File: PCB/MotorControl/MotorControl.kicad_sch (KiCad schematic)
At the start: 14 parts, among them J1 USB_C_Receptacle_USB2.0_14P, J2 Conn_02x05_Top_Bottom, J3 Conn_01x06, J4 Conn_01x03, SW1 SW_Push, U1 STM32L031K6Tx, U2 TC1262-33

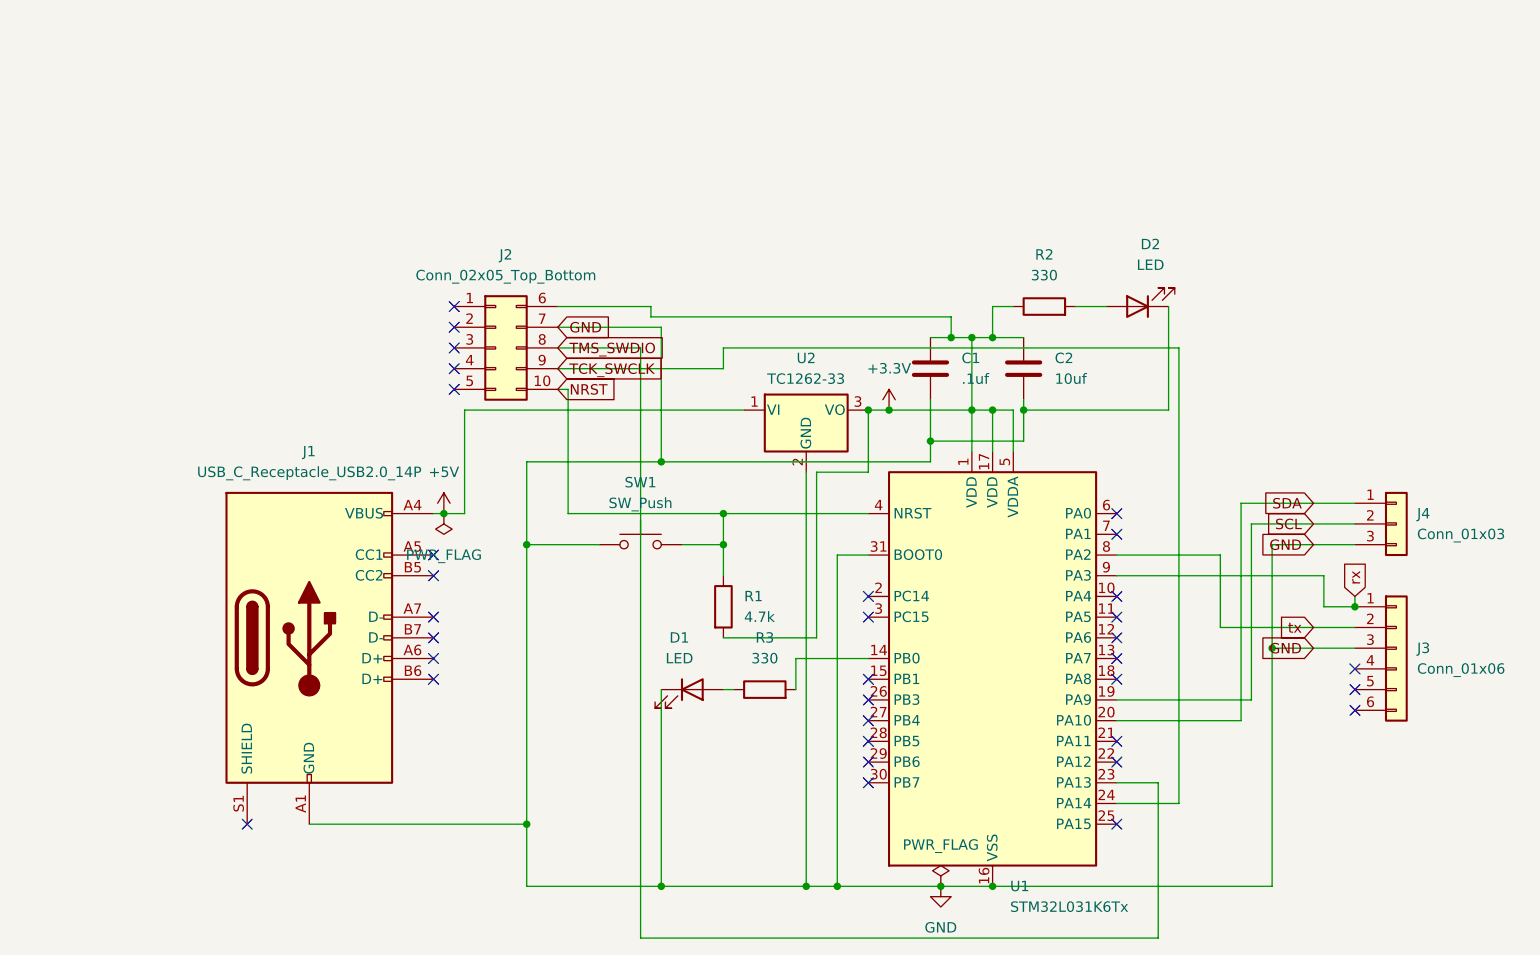
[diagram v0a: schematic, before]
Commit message: wasd
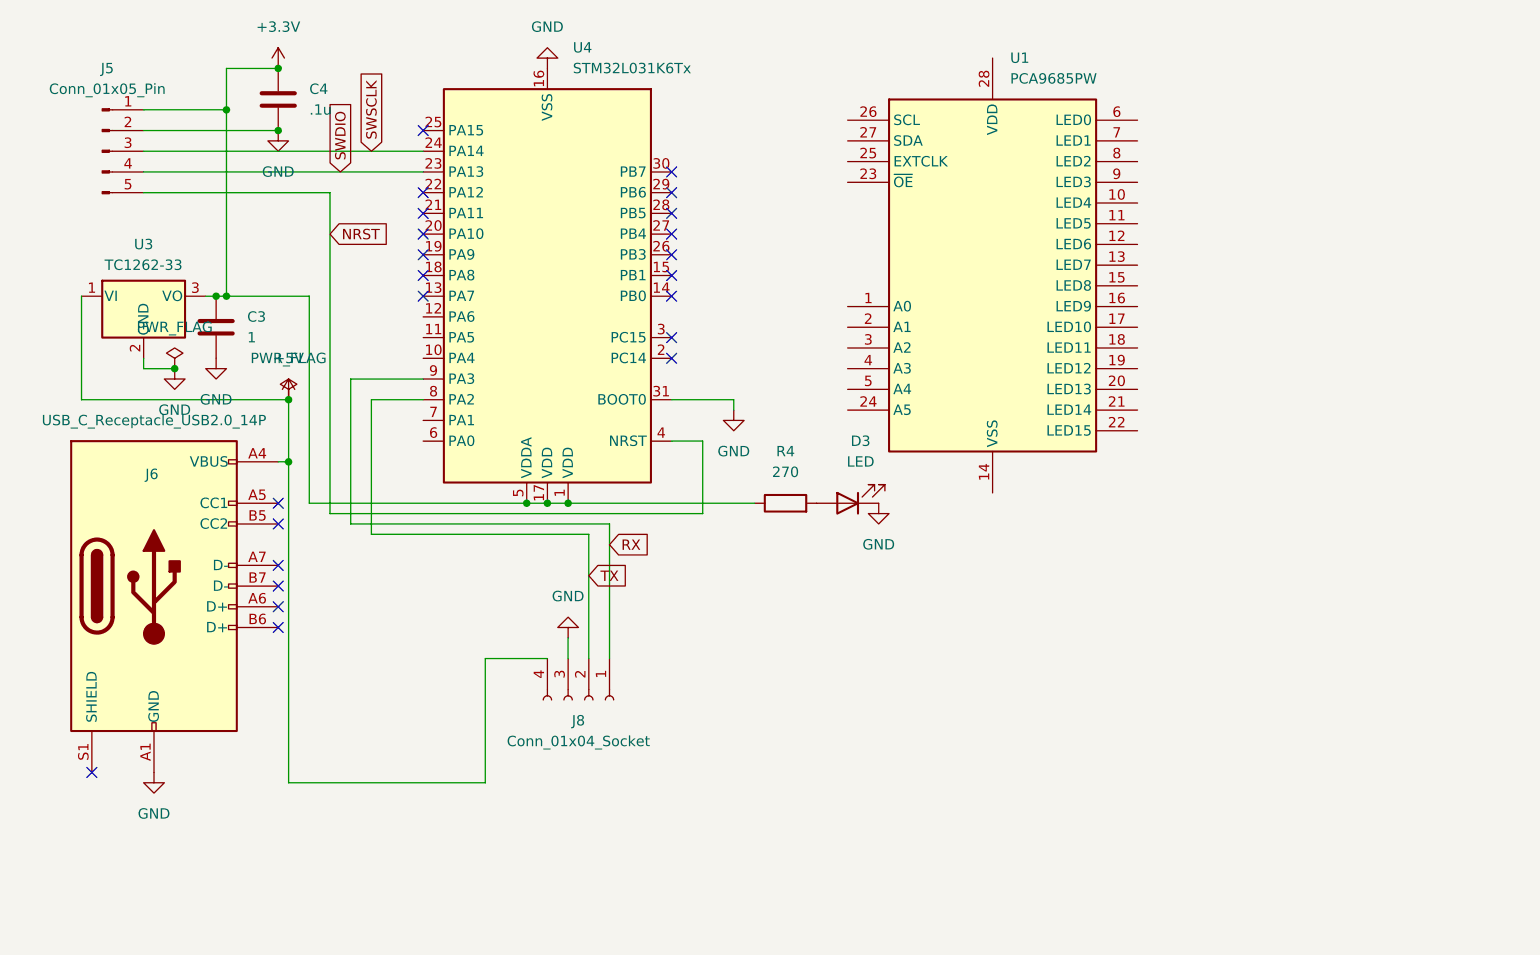
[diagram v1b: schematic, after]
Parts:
- removed C1: .1uf, Capacitor_SMD:C_0805_2012Metric_Pad1.18x1.45mm_HandSolder, symbol Device:C
- removed C2: 10uf, Capacitor_SMD:C_0805_2012Metric_Pad1.18x1.45mm_HandSolder, symbol Device:C
- removed D1, D2: LED, LED_SMD:LED_0805_2012Metric_Pad1.15x1.40mm_HandSolder, symbol Device:LED
- removed J1: USB_C_Receptacle_USB2.0_14P, Connector_USB:USB_C_Receptacle_GCT_USB4085, symbol Connector:USB_C_Receptacle_USB2.0_14P
- removed J2: Conn_02x05_Top_Bottom, Connector_PinHeader_2.54mm:PinHeader_2x05_P2.54mm_Vertical, symbol Connector_Generic:Conn_02x05_Top_Bottom
- removed J3: Conn_01x06, Connector_PinHeader_2.54mm:PinHeader_1x06_P2.54mm_Vertical, symbol Connector_Generic:Conn_01x06
- removed J4: Conn_01x03, Connector_PinHeader_2.54mm:PinHeader_1x03_P2.54mm_Vertical, symbol Connector_Generic:Conn_01x03
- removed R1: 4.7k, Resistor_SMD:R_0805_2012Metric_Pad1.20x1.40mm_HandSolder, symbol Device:R
- removed R2, R3: 330, Resistor_SMD:R_0805_2012Metric_Pad1.20x1.40mm_HandSolder, symbol Device:R
- removed SW1: SW_Push, Button_Switch_THT:SW_PUSH_6mm_H4.3mm, symbol Switch:SW_Push
- removed U1: STM32L031K6Tx, Package_QFP:LQFP-32_7x7mm_P0.8mm, symbol MCU_ST_STM32L0:STM32L031K6Tx
- removed U2: TC1262-33, Package_TO_SOT_SMD:SOT-223-3_TabPin2, symbol Regulator_Linear:TC1262-33
- added C3: 1, Capacitor_SMD:C_0504_1310Metric_Pad0.83x1.28mm_HandSolder, symbol Device:C
- added C4: .1u, Capacitor_SMD:C_0504_1310Metric_Pad0.83x1.28mm_HandSolder, symbol Device:C
- added D3: LED, LED_SMD:LED_1206_3216Metric_Pad1.42x1.75mm_HandSolder, symbol Device:LED
- added J5: Conn_01x05_Pin, Connector_PinHeader_1.00mm:PinHeader_1x05_P1.00mm_Vertical, symbol Connector:Conn_01x05_Pin
- added J6: USB_C_Receptacle_USB2.0_14P, Connector_USB:USB_C_Receptacle_GCT_USB4085, symbol Connector:USB_C_Receptacle_USB2.0_14P
- added J8: Conn_01x04_Socket, Connector_PinHeader_1.00mm:PinHeader_1x04_P1.00mm_Horizontal, symbol Connector:Conn_01x04_Socket
- added R4: 270, Resistor_SMD:R_0805_2012Metric_Pad1.20x1.40mm_HandSolder, symbol Device:R
- added U1: PCA9685PW, Package_SO:TSSOP-28_4.4x9.7mm_P0.65mm, symbol Driver_LED:PCA9685PW
- added U3: TC1262-33, Package_TO_SOT_SMD:SOT-223-3_TabPin2, symbol Regulator_Linear:TC1262-33
- added U4: STM32L031K6Tx, Package_QFP:LQFP-32_7x7mm_P0.8mm, symbol MCU_ST_STM32L0:STM32L031K6Tx
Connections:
- net +3.3V: now also C3.1, C4.1, J5.1 (Pin_1), R4.1, U3.3 (VO), U4.1 (VDD), U4.17 (VDD), U4.5 (VDDA)
- net +5V: now also J6.A4 (VBUS), J6.A9 (VBUS), J6.B4 (VBUS), J6.B9 (VBUS), J8.4 (Pin_4), U3.1 (VI)
- net GND: now also C3.2, C4.2, D3.1 (K), J5.2 (Pin_2), J6.A1 (GND), J6.A12 (GND), J6.B1 (GND), J6.B12 (GND), J8.3 (Pin_3), U3.2 (GND), U4.16 (VSS), U4.31 (BOOT0), U4.32 (VSS)
- net NRST: now also J5.5 (Pin_5), U4.4 (NRST)
- new net: D3.2 (A), R4.2
- new net RX: J8.1 (Pin_1), U4.9 (PA3)
- new net SWDIO: J5.4 (Pin_4), U4.23 (PA13)
- new net SWSCLK: J5.3 (Pin_3), U4.24 (PA14)
- new net TX: J8.2 (Pin_2), U4.8 (PA2)
- no-connect marks 33 -> 23
